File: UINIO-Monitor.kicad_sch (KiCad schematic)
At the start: 59 parts, among them J1 Conn_01x08_Pin, J2 Conn_01x08_Pin, J3 Conn_01x04_Pin, J4 Conn_01x08_Pin, J7 Conn_01x08_Pin, P1 LCD_Pad_10Pin, P2 LCD_Pad_12Pin, P3 OLED_Pad_30Pin, P4 LCD_Pad_13Pin, P5 LCD_Pad_12Pin, U1 ME6211, U2 ME6211, U3 XC6206PxxxMR, U4 ME6211, U5 ME6211

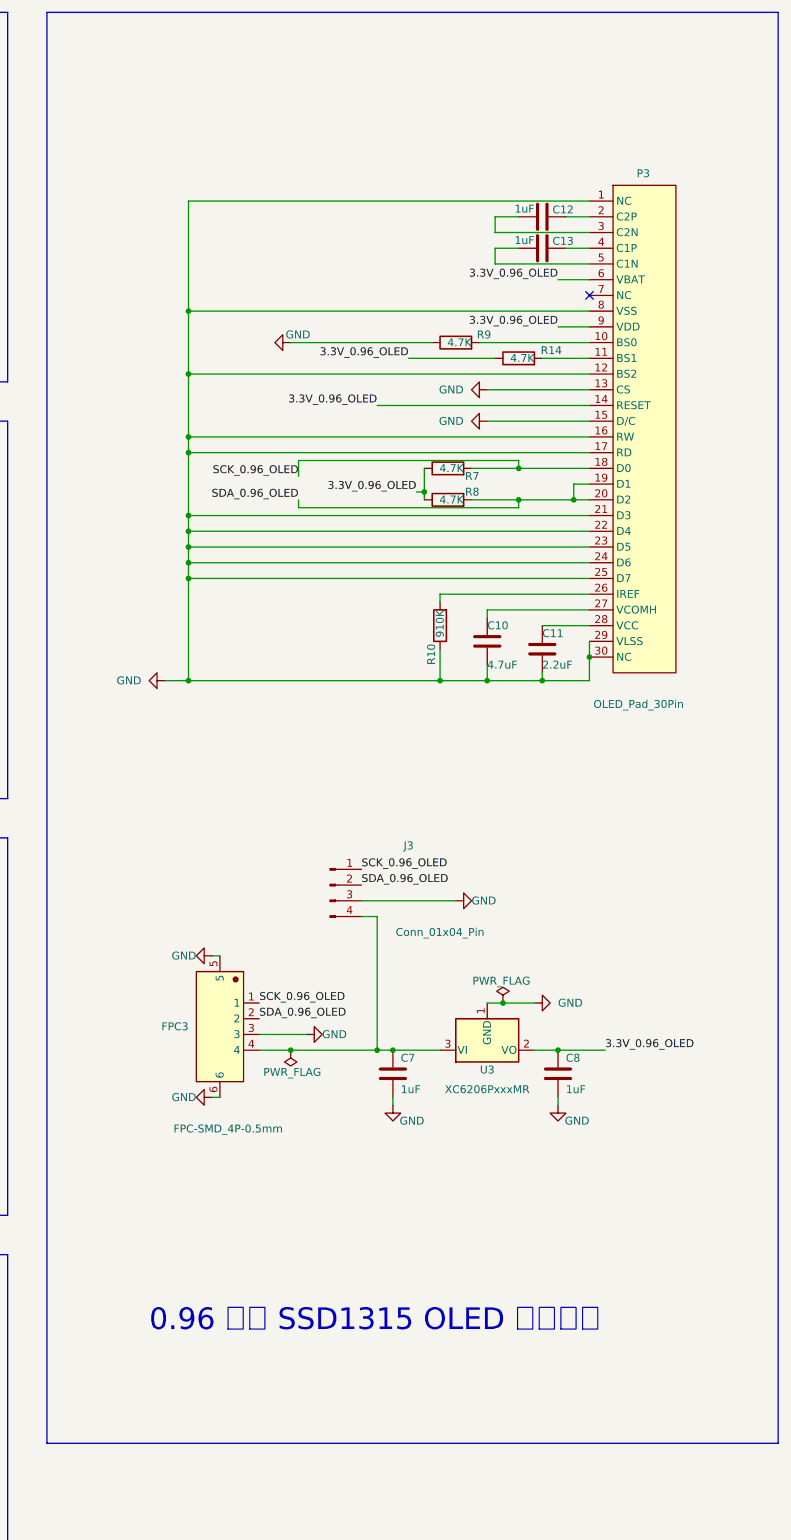
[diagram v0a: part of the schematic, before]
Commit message: Update PCB.
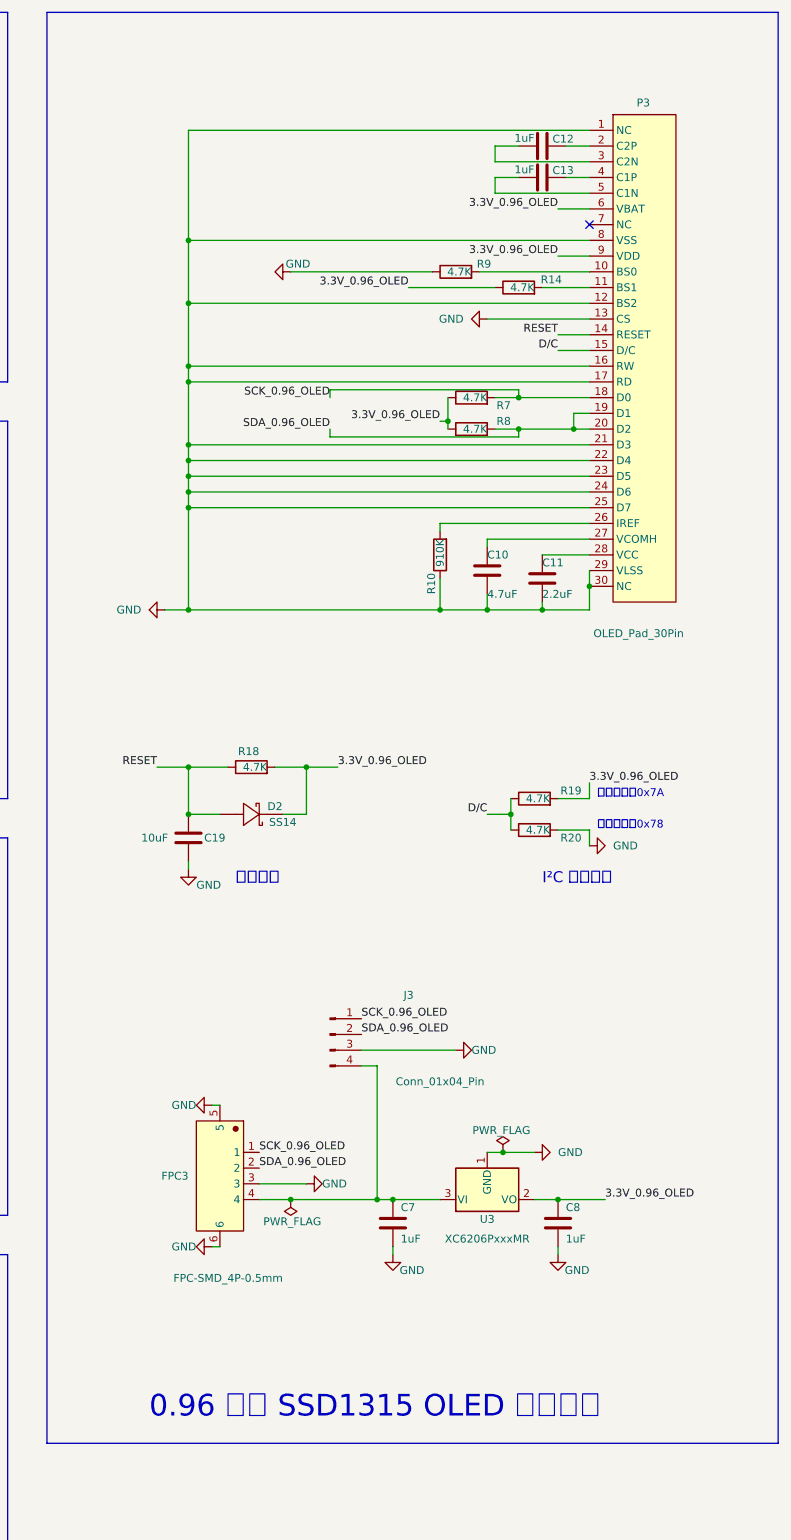
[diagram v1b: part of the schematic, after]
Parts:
- added C19: 10uF, Capacitor_SMD:C_0402_1005Metric, symbol Device:C
- added D2: SS14, Uinio:SMA_L4.3-W2.5-LS5.0-RD, symbol Uinio:SS14
- added R18, R19, R20: 4.7K, Resistor_SMD:R_0402_1005Metric, symbol Device:R
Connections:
- net 3.3V_0.96_OLED: now also D2.1 (K), R18.2, R19.2; no longer P3.14 (RESET)
- net GND: now also C19.2, R20.2; no longer P3.15 (D/C)
- new net D/C: P3.15 (D/C), R19.1, R20.1
- new net RESET: C19.1, D2.2 (A), P3.14 (RESET), R18.1
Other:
- note added: "I²C 地址选择"
- note added: "上拉地址：0x7A"
- note added: "下拉地址：0x78"
- note added: "复位逻辑"
- moved on the sheet: C10, C11, C12, C13, C7, C8, FPC3, J3, P3, R10, R14, R7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
